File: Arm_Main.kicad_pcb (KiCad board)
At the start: 2 copper layers, 99 x 78.5 mm, 41 parts, among them IC1 TLP559_F_, IC2 TLP559_F_, J1 Conn_01x02_Pin, J2 Conn_01x03_Pin, J3 Conn_01x03_Pin, J4 Conn_01x03_Pin, J5 Conn_01x03_Socket, SW4 SW_SPST, SW5 SW_SPST, SW6 SW_SPST, U1 RASPBERRY_PI_ZERO_2_W, U2 TLP2531, U3 ADuM121N

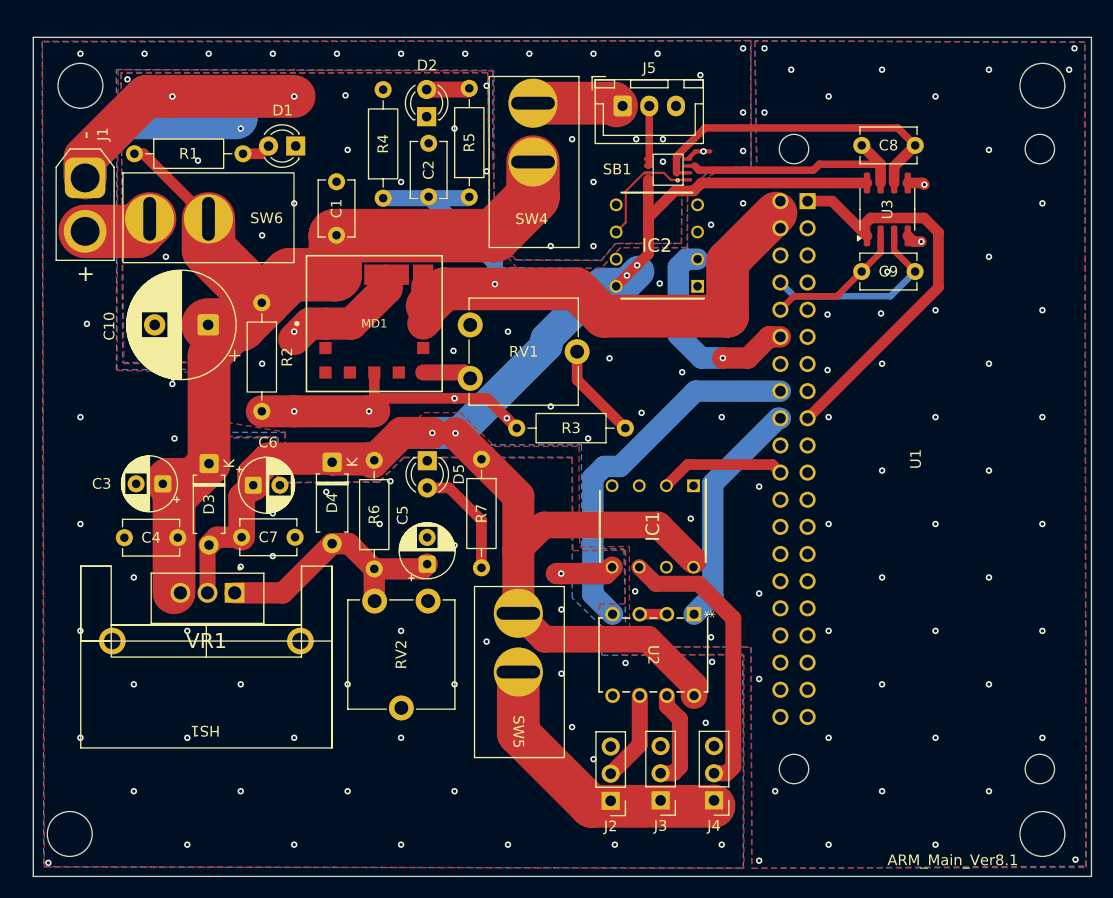
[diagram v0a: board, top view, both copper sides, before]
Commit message: ver9
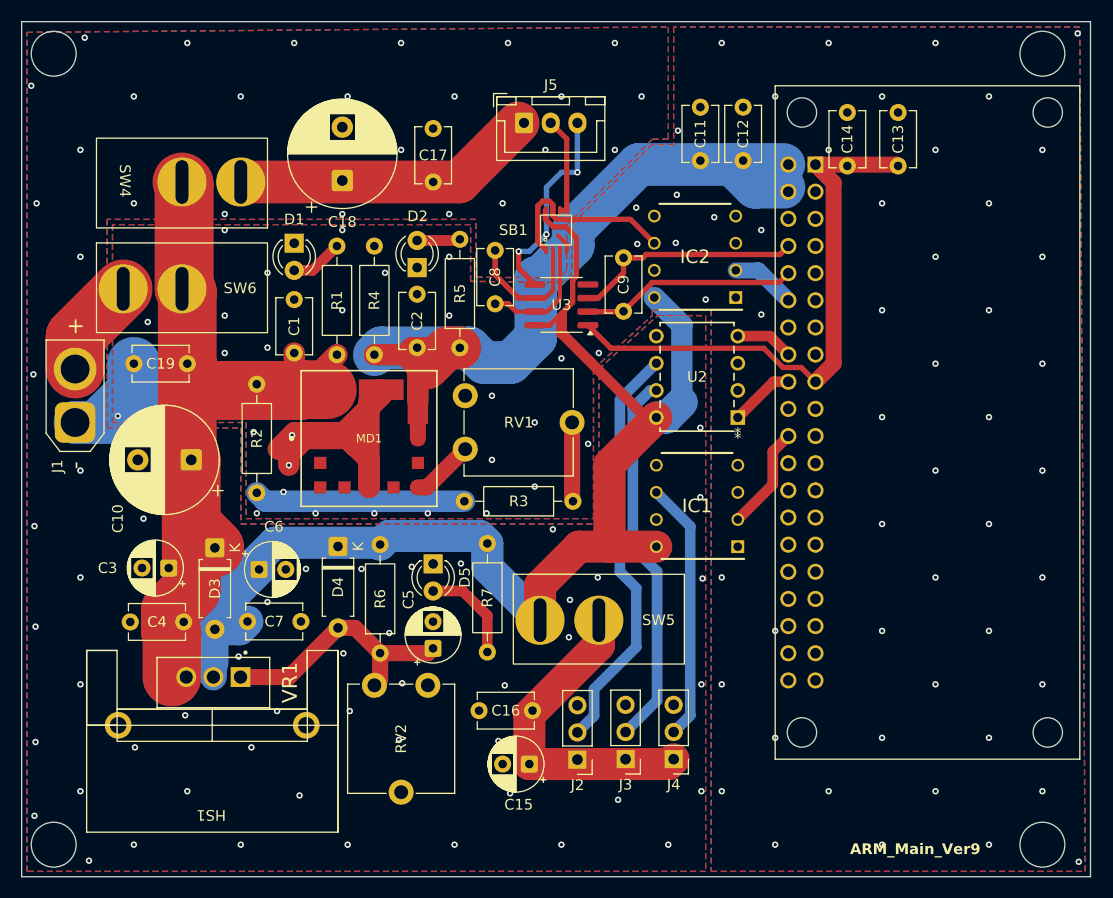
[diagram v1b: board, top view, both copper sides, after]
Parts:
- added C11: 10u, Capacitor_THT:C_Disc_D5.1mm_W3.2mm_P5.00mm, F.Cu at (163.0, 61.0)
- added C12: 0.1u, Capacitor_THT:C_Disc_D5.1mm_W3.2mm_P5.00mm, F.Cu at (167.0, 61.0)
- added C13: 10u, Capacitor_THT:C_Disc_D5.1mm_W3.2mm_P5.00mm, F.Cu at (181.5, 61.5)
- added C14: 0.1u, Capacitor_THT:C_Disc_D5.1mm_W3.2mm_P5.00mm, F.Cu at (176.8, 61.5)
- added C15: 470u, Capacitor_THT:CP_Radial_D5.0mm_P2.50mm, F.Cu at (147.0, 122.5)
- added C16: 0.1u, Capacitor_THT:C_Disc_D5.1mm_W3.2mm_P5.00mm, F.Cu at (147.3, 117.5)
- added C17: 0.1u, Capacitor_THT:C_Disc_D5.1mm_W3.2mm_P5.00mm, F.Cu at (138.0, 68.0)
- added C18: 1000u, Capacitor_THT:CP_Radial_D10.0mm_P5.00mm, F.Cu at (129.5, 67.9)
- added C19: 0.1u, Capacitor_THT:C_Disc_D5.1mm_W3.2mm_P5.00mm, F.Cu at (115.0, 85.0)
- moved C8 37.4 mm to (143.8, 79.4), turned to 90 degrees
- moved SW4 32.9 mm to (114.5, 68.0), turned to 180 degrees
- moved U3 31.8 mm to (150.0, 79.5), turned to 180 degrees
- moved R1 26.7 mm to (129.0, 84.2), turned to 90 degrees
- moved J1 22.9 mm to (104.5, 90.5), turned to 90 degrees
- moved C9 22.6 mm to (155.8, 80.1), turned to 90 degrees
- moved U2 18.8 mm to (166.5, 90.0), turned to 180 degrees
- moved R4 14.7 mm to (132.5, 84.2)
- moved C2 14.2 mm to (136.5, 83.5)
- moved D2 14.1 mm to (136.5, 76.0)
- moved R5 14.1 mm to (140.5, 83.5)
- moved C10 12.7 mm to (115.4, 94.0)
- moved SB1 11.9 mm to (149.5, 72.5), turned to 90 degrees
- moved C1 11.7 mm to (125.0, 84.0)
- moved MD1 10.8 mm to (132.0, 92.0)
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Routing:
- net +5V_Analog: track 166.3 -> 135.6 mm, vias 4 -> 0
- net Net-(J2-Pin_2): track 8.43 -> 38.9 mm
- net Net-(U1-GPIO23/GPIO_GEN4): track 34.4 -> 5.45 mm
- net Net-(J3-Pin_2): track 9.21 -> 35.4 mm
- net Batte: track 95.5 -> 72.2 mm
- net Net-(J5-Pin_1): track 7.94 -> 28.2 mm
- net Net-(SB1-A1): track 31.0 -> 12.7 mm
- net Net-(U1-GPIO24/GPIO_GEN5): track 21.8 -> 6.12 mm
- net Net-(U1-3V3_1): track 37.7 -> 53.0 mm
- net Net-(IC2-ANODE): track 19.7 -> 6.08 mm, vias 1 -> 0
- net GNDA: track 93.5 -> 106.1 mm, vias 153 -> 156
- net Net-(SB1-Y2): track 22.7 -> 11.4 mm
- net +5V_Digital: track 67.2 -> 77.1 mm, vias 1 -> 0
- net Net-(U1-GPIO15/RXD0): track 13.1 -> 20.3 mm
- net Net-(IC2-COLLECTER): track 11.0 -> 17.7 mm
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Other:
- board size 99 x 78.5 mm -> 100 x 80 mm
- board text added: "ARM_Main_Ver9"
- board text removed: "ARM_Main_Ver8.1"
